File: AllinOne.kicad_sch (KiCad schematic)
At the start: 15 parts, among them P1 USB_C_Plug_USB2.0, SW1 SW_Push, U1 AT90USB1286-AU, Y1 16MHz

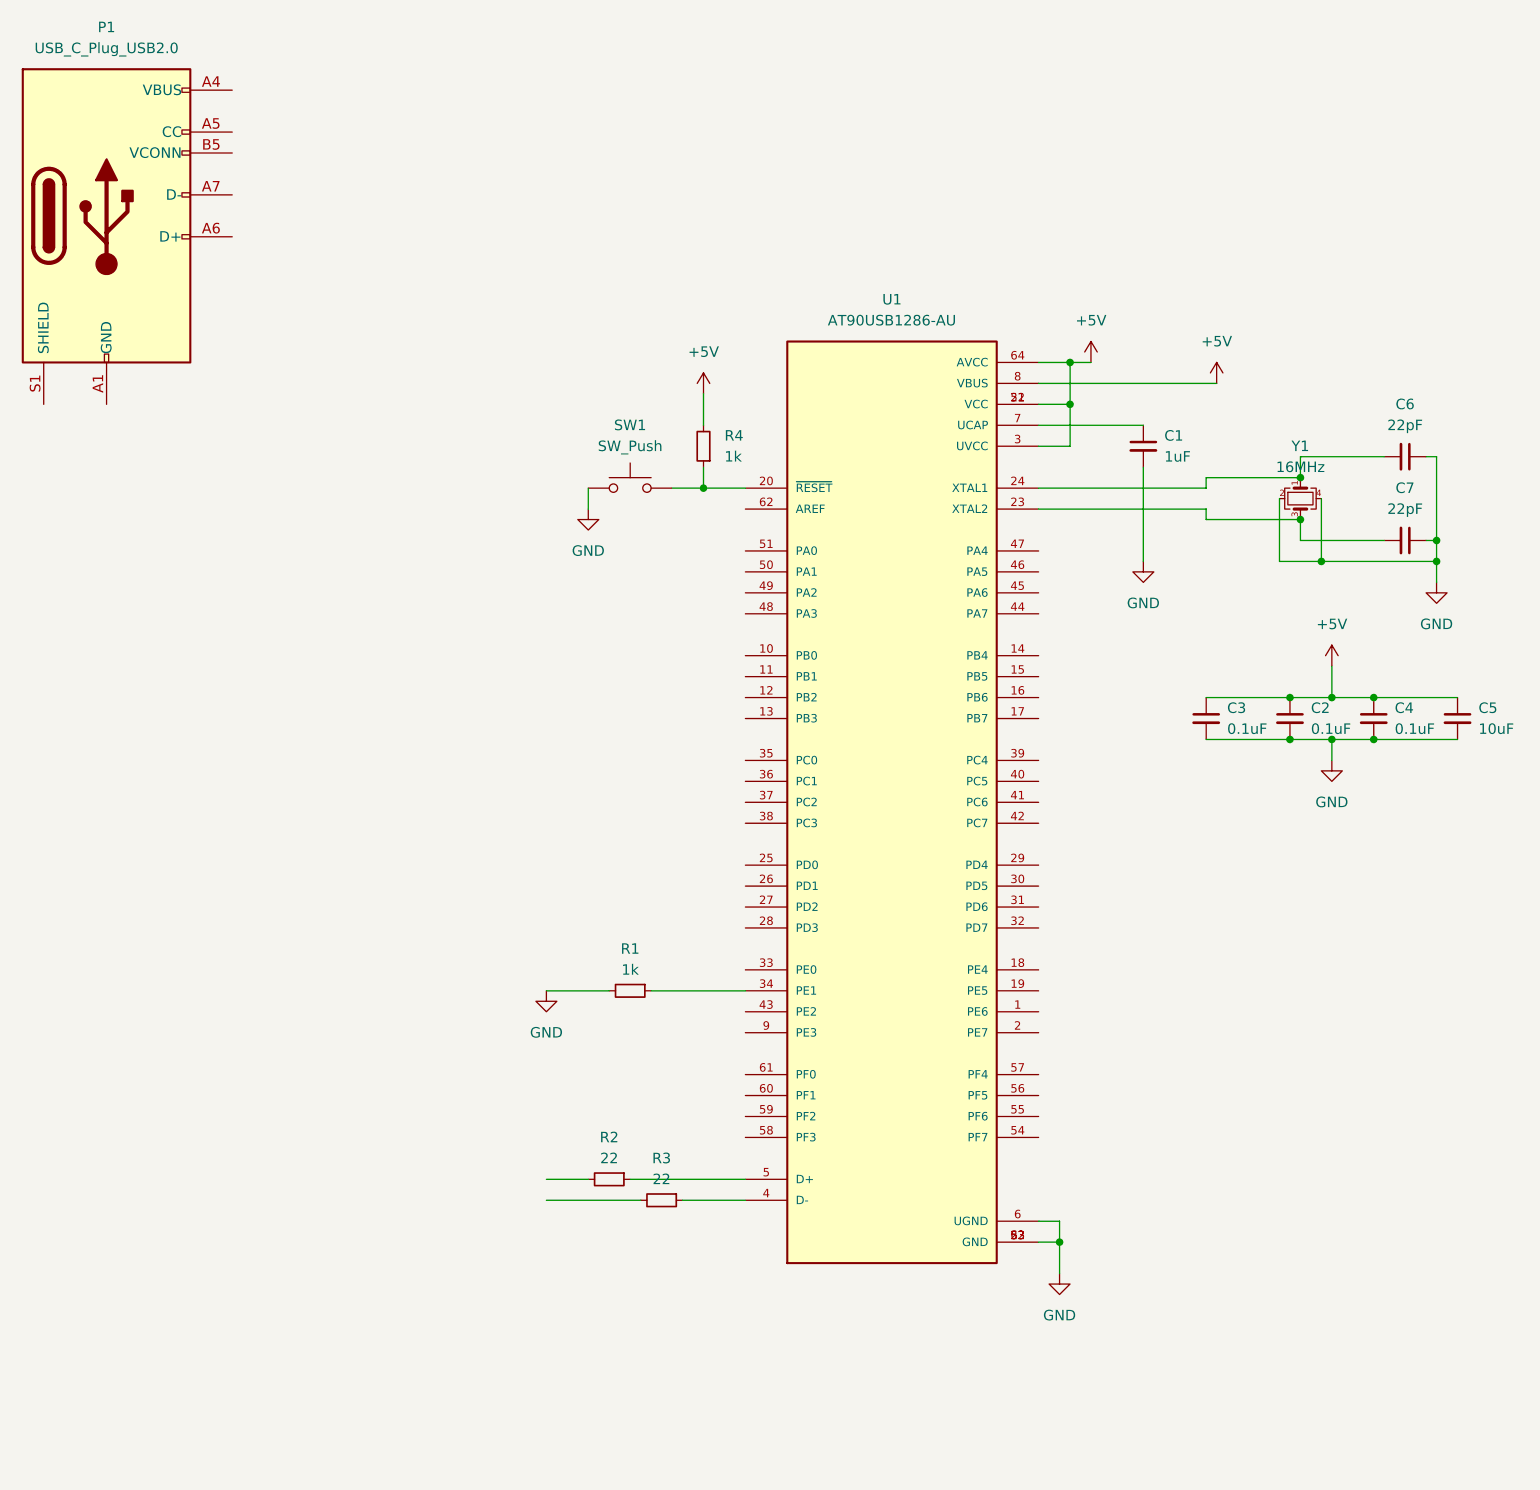
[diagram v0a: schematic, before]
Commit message: Schematic all done
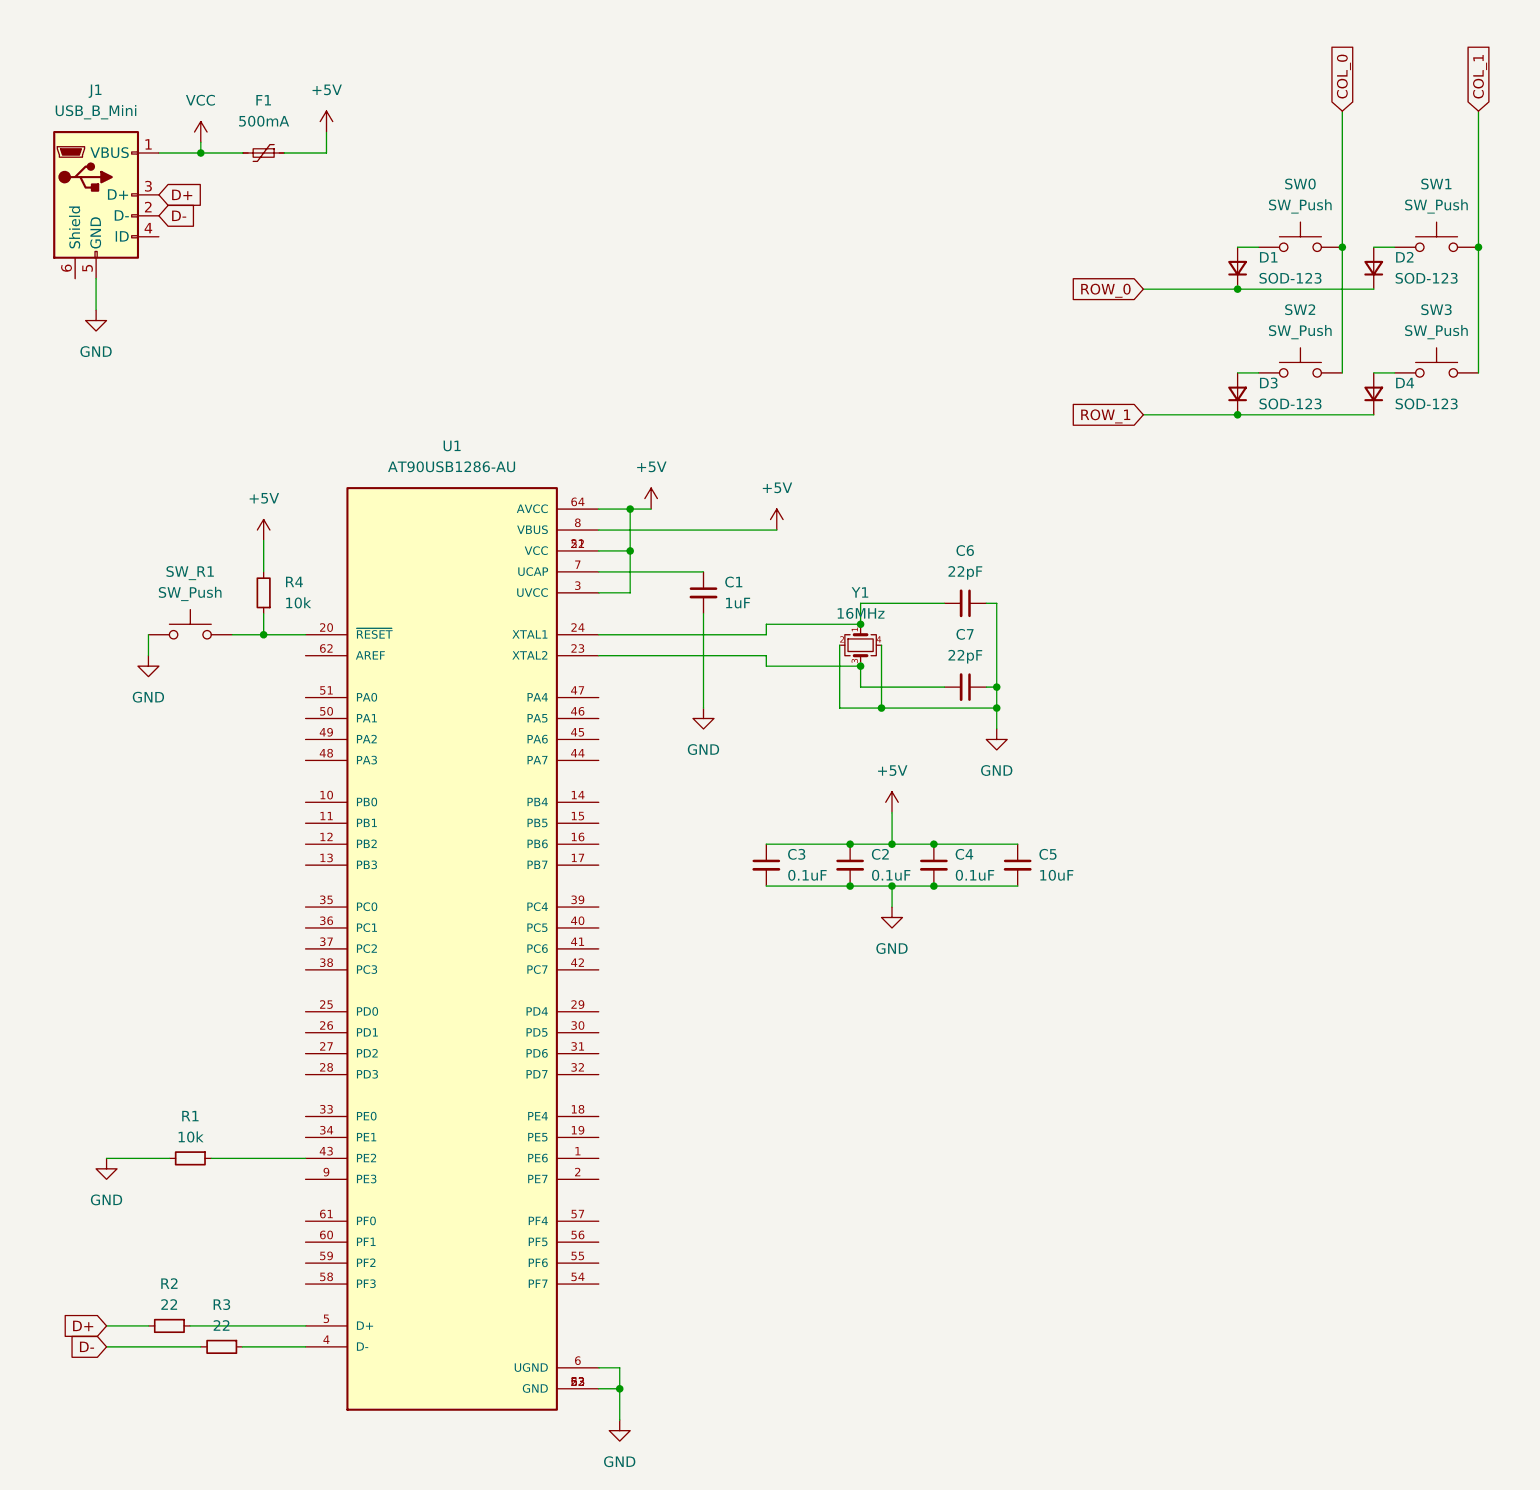
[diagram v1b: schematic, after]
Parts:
- removed P1: USB_C_Plug_USB2.0, symbol Connector:USB_C_Plug_USB2.0
- added D1, D2, D3, D4: SOD-123, Diode_SMD:D_SOD-123, symbol Device:D_Small
- added F1: 500mA, Fuse:Fuse_1206_3216Metric, symbol Device:Polyfuse_Small
- added J1: USB_B_Mini, Connector_USB:USB3_A_Molex_48393-001, symbol Connector:USB_B_Mini
- added SW0, SW1, SW2, SW3: SW_Push, Button_Switch_Keyboard:SW_Cherry_MX_1.00u_PCB, symbol Switch:SW_Push
- C1, C2, C3, C4, C5, C6, C7: footprint (none) -> Capacitor_SMD:C_0805_2012Metric
- R1, R4: value 1k -> 10k; footprint (none) -> Resistor_SMD:R_0805_2012Metric
- R2, R3: footprint (none) -> Resistor_SMD:R_0805_2012Metric
- SW_R1: renamed from SW1; footprint (none) -> Button_Switch_THT:SW_PUSH_6mm
- U1: footprint (none) -> CustomMCUs:AT90USB1286-AU
- Y1: footprint (none) -> Crystal:Crystal_SMD_3225-4Pin_3.2x2.5mm
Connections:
- net +5V: now also F1.1
- net GND: now also J1.5 (GND)
- net D-: now reaches R3.2
- net D-: now also J1.2 (D-)
- net at R1.1: now also U1.43 (PE2); no longer U1.34 (PE1)
- net D+: now reaches R2.2
- net D+: now also J1.3 (D+)
- new net: D1.2 (A), SW0.1
- new net: D2.2 (A), SW1.1
- new net: D3.2 (A), SW2.1
- new net: D4.2 (A), SW3.1
- new net COL_0: SW0.2, SW2.2
- new net COL_1: SW1.2, SW3.2
- new net ROW_0: D1.1 (K), D2.1 (K)
- new net ROW_1: D3.1 (K), D4.1 (K)
- new net VCC: F1.2, J1.1 (VBUS)
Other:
- moved on the sheet: C1, C2, C3, C4, C5, C6, C7, R1, R2, R3, R4, SW_R1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
